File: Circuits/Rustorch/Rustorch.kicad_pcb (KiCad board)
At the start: 4 copper layers, 95 x 72 mm, 57 parts, among them CN1 USB_C_Receptacle_USB2.0_16P, CN2 OLED_128x64_IIC, Q1 2SC1815, Q2 2SC1815, Q3 2SC1815, Q4 2SC1815, SW1 ToggleSW 3P, SW2 RESET, SW3 SW_BOOT, SW4 SW_UP, SW5 SW_LEFT, SW6 SW_RIGHT, SW7 SW_DOWN, SW8 SW_A, SW9 SW_B, U1 ESP32-C6-WROOM-1, U2 BA033CC0T, U3 OSL10561-L*, U4 OSL10561-L*, U5 OSL10561-L*, U6 OSL10561-L*

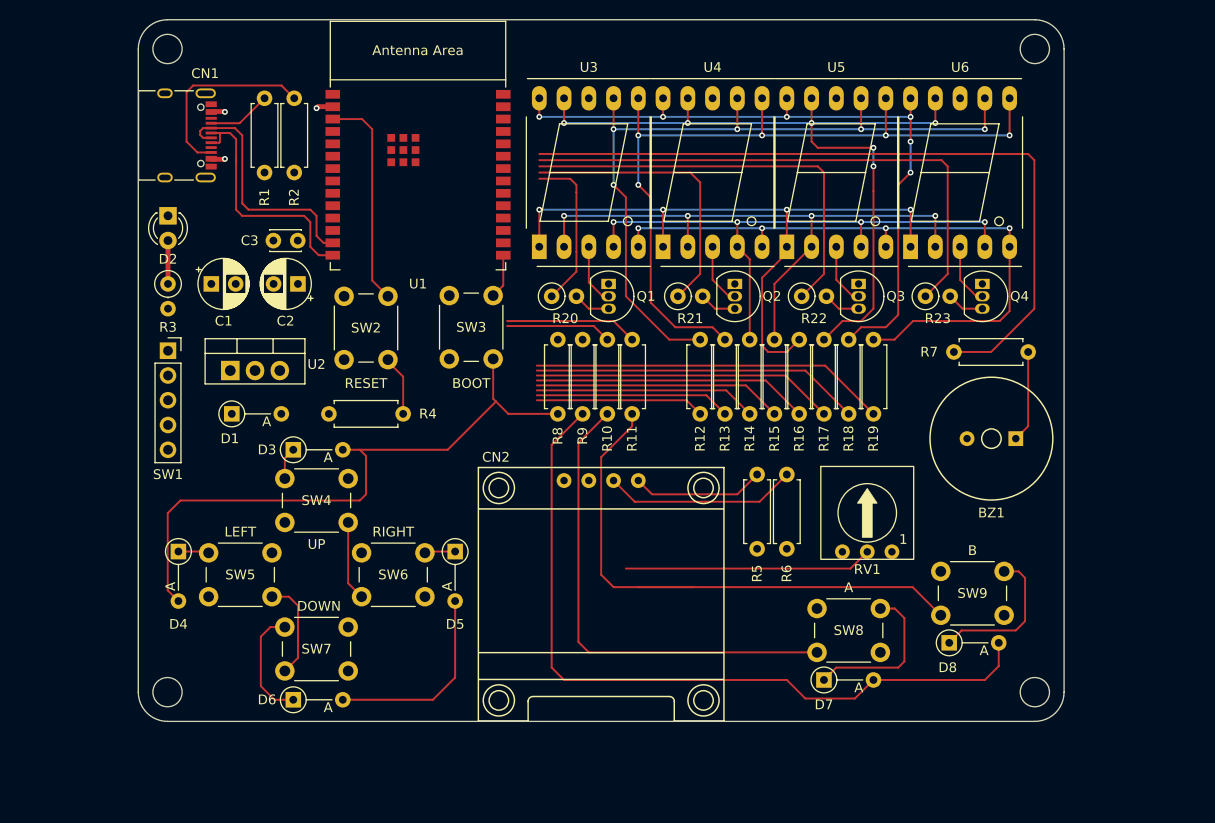
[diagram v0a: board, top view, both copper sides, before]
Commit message: (Rustorch) 配線作業 (一通り接続完了した状態)
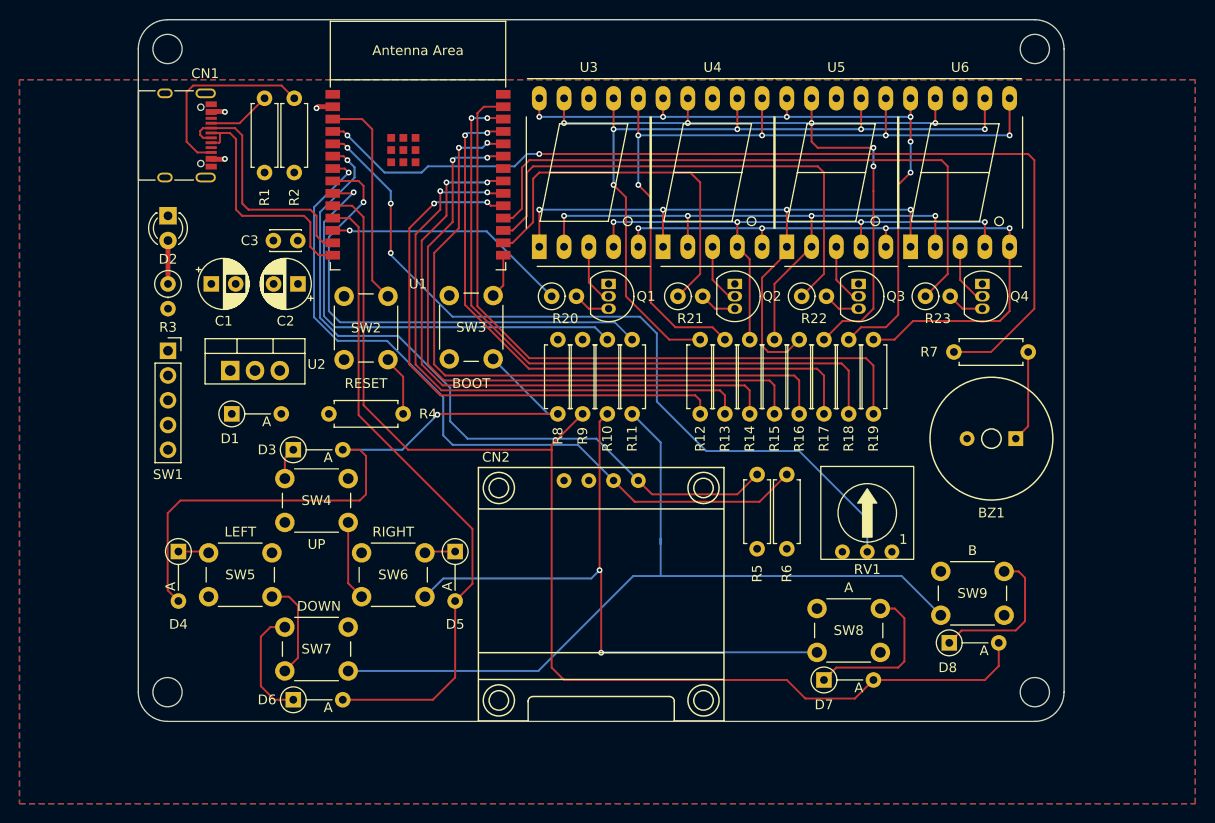
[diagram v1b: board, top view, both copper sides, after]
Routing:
- net SDA: track 13.6 -> 74.8 mm, vias 0 -> 1
- net SCL: track 19.8 -> 77.9 mm, vias 0 -> 1
- net Net-(U1-MTDI/GPIO5/ADC1_CH5): track 25.5 -> 82.1 mm, vias 0 -> 3
- net KEY_IN2: track 20.3 -> 67.3 mm
- net KEY_IN3_IO8: track 78.3 -> 122.5 mm
- net 7SEG_E: track 28.3 -> 69.7 mm, vias 0 -> 2
- net 7SEG_D: track 25.6 -> 66.7 mm, vias 0 -> 2
- net 7SEG_A: track 17.5 -> 57.8 mm, vias 0 -> 2
- net 7SEG_B: track 20.1 -> 60.4 mm, vias 0 -> 2
- net 7SEG_C: track 22.8 -> 62.8 mm, vias 0 -> 2
- net KEY_OUT2: track 13.6 -> 50.0 mm, vias 0 -> 1
- net KEY_OUT1: track 10.9 -> 46.2 mm, vias 0 -> 1
- net 7SEG_G: track 33.8 -> 68.5 mm, vias 0 -> 2
- net 7SEG_DP: track 36.6 -> 70.9 mm
- net 7SEG_F: track 31.1 -> 65.3 mm, vias 0 -> 2
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- added copper zone on B.Cu, net GND
- added copper zone on F.Cu, net GND
